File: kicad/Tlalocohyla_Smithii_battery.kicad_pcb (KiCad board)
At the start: 2 copper layers, 85.2 x 29.4 mm, 3 parts

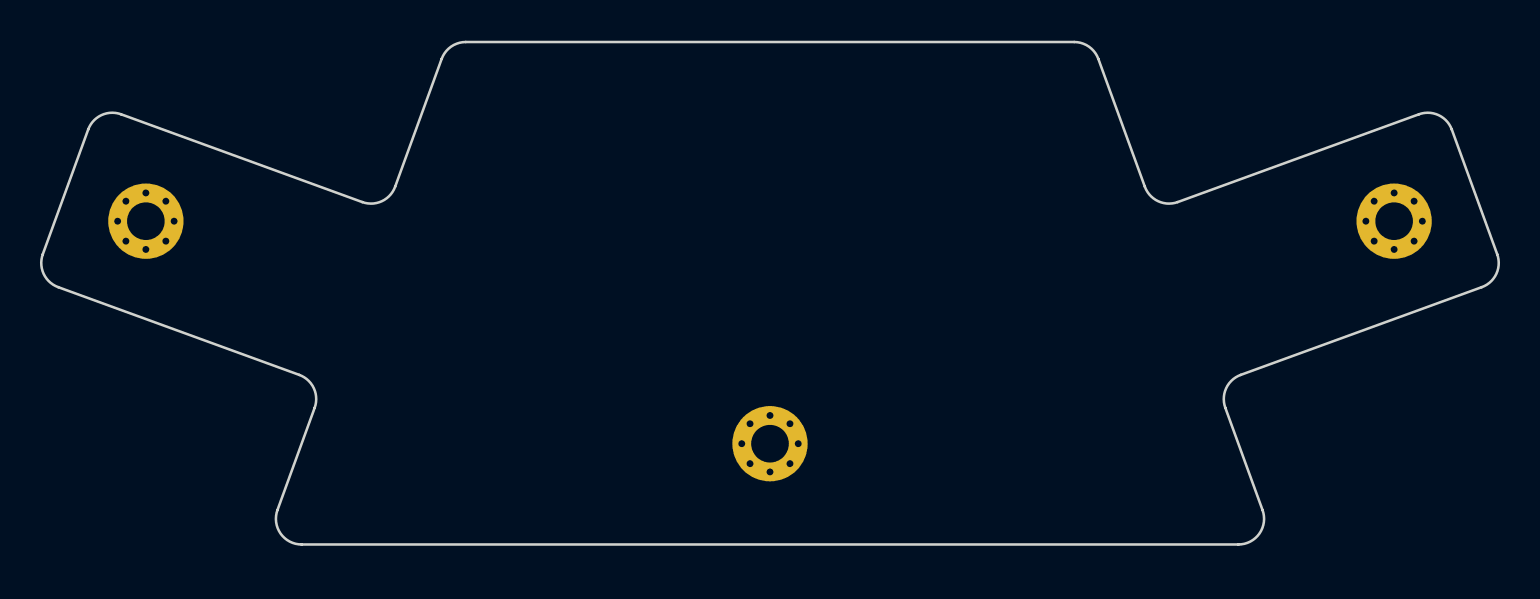
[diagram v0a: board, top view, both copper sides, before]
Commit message: Add filled zone
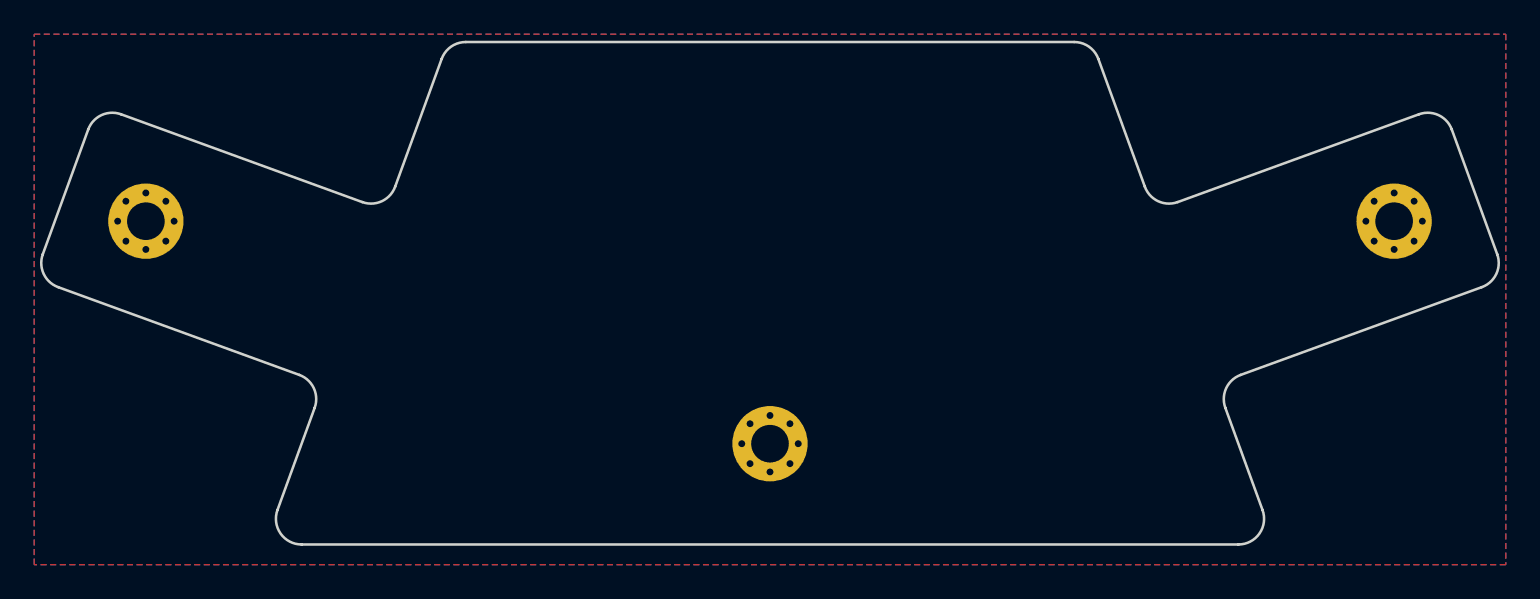
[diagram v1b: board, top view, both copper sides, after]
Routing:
- added copper zone on B.Cu, net (none)
- added copper zone on F.Cu, net (none)
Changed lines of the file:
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@@
   (gr_line (start 132.221213 98.455283) (end 167.778787 98.455283) (layer "Edge.Cuts") (width 0.15))
   (gr_arc (start 173.829848 107.809025) (mid 172.682891 107.758948) (end 171.90728 106.912517) (layer "Edge.Cuts") (width 0.15))
+  (zone (net 0) (net_name "") (layers F&B.Cu) (hatch edge 0.508)
+    (connect_pads (clearance 0.508))
+    (min_thickness 0.254) (filled_areas_thickness no)
+    (fill yes (thermal_gap 0.508) (thermal_bridge_width 0.508))
+    (polygon
+      (pts
+        (xy 193 129)
+        (xy 107 129)
+        (xy 107 98)
+        (xy 193 98)
+      )
+    )
+  )
 )
